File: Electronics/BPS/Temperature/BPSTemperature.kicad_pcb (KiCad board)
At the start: 2 copper layers, 75 x 65 mm, 59 parts, among them J1 Conn_02x10_Counter_Clockwise, J2 Logic Analyzer, J3 Conn_02x06_Counter_Clockwise, J4 Conn_02x06_Counter_Clockwise, SW1 SW_DIP_x06, U1 LTC2983

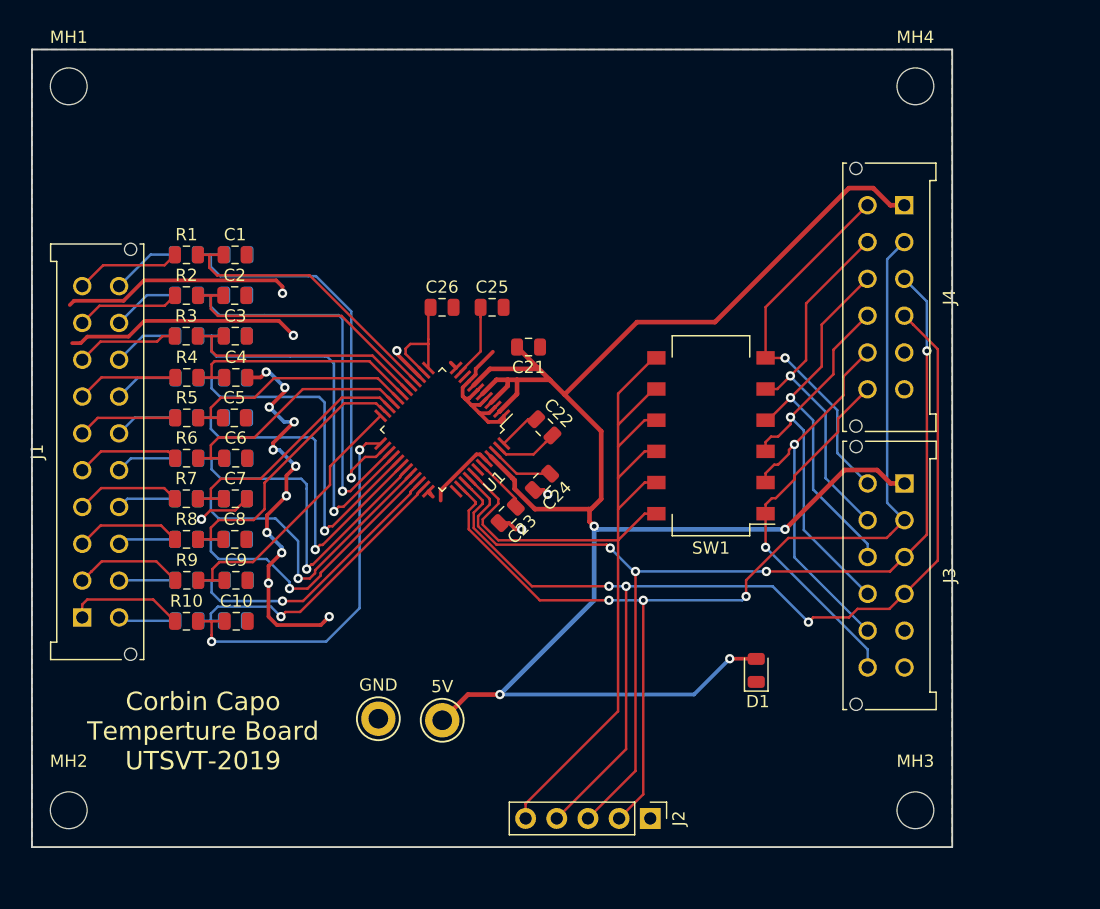
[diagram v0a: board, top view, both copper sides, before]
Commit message: Made edits to temperature board. Finalized boards.
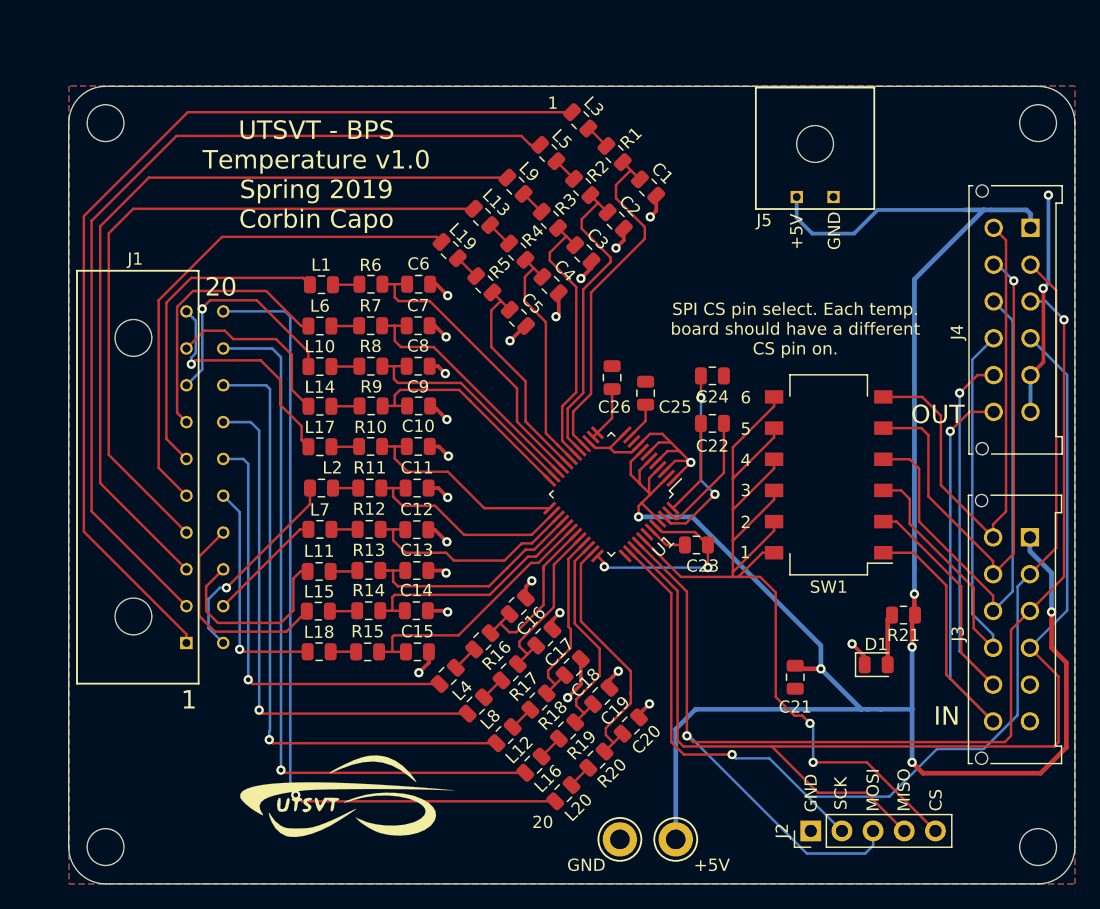
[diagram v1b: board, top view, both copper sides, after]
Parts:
- removed 5V: TestPoint, TestPoint:TestPoint_Keystone_5005-5009_Compact
- added +5V: TestPoint, TestPoint:TestPoint_Keystone_5005-5009_Compact, F.Cu at (102.5, 131.4)
- added G***: LOGO, UTSVT_Special:UTSVT_Logo_Symbol, F.Cu at (75.4, 128.0)
- added G***: LOGO, UTSVT_Special:Hallock_Image, B.Cu at (83.2, 100.8)
- added J5: Conn_01x02, UTSVT_Connectors:43650-0202_01x02_Microfit 3.0_horizontal, F.Cu at (109.0, 80.0)
- added L1: Ferrite_Bead, Inductor_SMD:L_0805_2012Metric, F.Cu at (73.6, 86.2)
- added L10: Ferrite_Bead, Inductor_SMD:L_0805_2012Metric, F.Cu at (73.5, 92.8)
- added L11: Ferrite_Bead, Inductor_SMD:L_0805_2012Metric, F.Cu at (73.4, 109.5)
- added L12: Ferrite_Bead, Inductor_SMD:L_0805_2012Metric, F.Cu at (88.5, 122.9)
- added L13: Ferrite_Bead, Inductor_SMD:L_0805_2012Metric, F.Cu at (86.7, 80.6)
- added L14: Ferrite_Bead, Inductor_SMD:L_0805_2012Metric, F.Cu at (73.5, 96.1)
- added L15: Ferrite_Bead, Inductor_SMD:L_0805_2012Metric, F.Cu at (73.3, 112.8)
- added L16: Ferrite_Bead, Inductor_SMD:L_0805_2012Metric, F.Cu at (90.9, 125.3)
- added L17: Ferrite_Bead, Inductor_SMD:L_0805_2012Metric, F.Cu at (73.5, 99.4)
- added L18: Ferrite_Bead, Inductor_SMD:L_0805_2012Metric, F.Cu at (73.4, 116.1)
- added L19: Ferrite_Bead, Inductor_SMD:L_0805_2012Metric, F.Cu at (84.0, 83.3)
- added L2: Ferrite_Bead, Inductor_SMD:L_0805_2012Metric, F.Cu at (73.6, 102.7)
- added L20: Ferrite_Bead, Inductor_SMD:L_0805_2012Metric, F.Cu at (93.3, 127.6)
- added L3: Ferrite_Bead, Inductor_SMD:L_0805_2012Metric, F.Cu at (94.7, 72.8)
- added L4: Ferrite_Bead, Inductor_SMD:L_0805_2012Metric, F.Cu at (83.9, 118.0)
- added L5: Ferrite_Bead, Inductor_SMD:L_0805_2012Metric, F.Cu at (92.1, 75.4)
- added L6: Ferrite_Bead, Inductor_SMD:L_0805_2012Metric, F.Cu at (73.5, 89.5)
- added L7: Ferrite_Bead, Inductor_SMD:L_0805_2012Metric, F.Cu at (73.5, 106.1)
- added L8: Ferrite_Bead, Inductor_SMD:L_0805_2012Metric, F.Cu at (86.2, 120.5)
- added L9: Ferrite_Bead, Inductor_SMD:L_0805_2012Metric, F.Cu at (89.4, 78.1)
- added R21: 1.55k, Resistor_SMD:R_0805_2012Metric, F.Cu at (121.0, 113.1)
- C11, C12, C13, C14, C15, C16, C17, C18, C19, C20, R11, R12, R13, R14, R15, R16, R17, R18, R19, R20: moved to F.Cu
- J1: footprint Connector_Molex:Molex_Micro-Fit_3.0_43045-2012_2x10_P3.00mm_Vertical -> UTSVT_Connectors:02x10_Microfit_3.0_horizontal
- moved R1 35.8 mm to (97.5, 75.5), turned to 315 degrees
- moved R20 35.2 mm to (96.0, 124.9), turned to 45 degrees
- moved C21 34.6 mm to (112.2, 118.2), turned to 90 degrees
- moved C1 34.1 mm to (100.2, 78.2), turned to 315 degrees
- moved R2 33.4 mm to (94.8, 78.2), turned to 315 degrees
- moved C20 33.3 mm to (98.8, 122.1), turned to 45 degrees
- moved R19 33.3 mm to (93.6, 122.5), turned to 45 degrees
- moved C2 31.6 mm to (97.6, 80.9), turned to 315 degrees
- moved R18 31.6 mm to (91.3, 120.1), turned to 45 degrees
- moved C19 31.2 mm to (96.4, 119.7), turned to 45 degrees
- moved R3 31.1 mm to (92.2, 80.9), turned to 315 degrees
- moved R17 29.9 mm to (88.9, 117.8), turned to 45 degrees
- moved C18 29.4 mm to (94.1, 117.3), turned to 45 degrees
- moved C3 29.2 mm to (94.9, 83.6), turned to 315 degrees
- moved R4 28.8 mm to (89.6, 83.5), turned to 315 degrees
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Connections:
- D1 pad 2: +5V -> Net-(D1-Pad2)
- J1 pad 1: /CH10_LPF -> /CH1_LPF
- J1 pad 10: /CH1_LPF -> /CH10_LPF
- J1 pad 11: /CH20_LPF -> /CH11_LPF
- J1 pad 12: /CH19_LPF -> /CH12_LPF
- J1 pad 13: /CH18_LPF -> /CH13_LPF
- J1 pad 14: /CH17_LPF -> /CH14_LPF
- J1 pad 15: /CH16_LPF -> /CH15_LPF
- J1 pad 16: /CH15_LPF -> /CH16_LPF
- J1 pad 17: /CH14_LPF -> /CH17_LPF
- J1 pad 18: /CH13_LPF -> /CH18_LPF
- J1 pad 19: /CH12_LPF -> /CH19_LPF
- J1 pad 2: /CH9_LPF -> /CH2_LPF
- J1 pad 20: /CH11_LPF -> /CH20_LPF
- J1 pad 3: /CH8_LPF -> /CH3_LPF
- J1 pad 4: /CH7_LPF -> /CH4_LPF
- J1 pad 5: /CH6_LPF -> /CH5_LPF
- J1 pad 6: /CH5_LPF -> /CH6_LPF
- J1 pad 7: /CH4_LPF -> /CH7_LPF
- J1 pad 8: /CH3_LPF -> /CH8_LPF
- J1 pad 9: /CH2_LPF -> /CH9_LPF
- R1 pad 1: /CH1_LPF -> Net-(L3-Pad1)
- R10 pad 1: /CH10_LPF -> Net-(L17-Pad1)
- R11 pad 1: /CH11_LPF -> Net-(L2-Pad2)
- R12 pad 1: /CH12_LPF -> Net-(L7-Pad2)
- R13 pad 1: /CH13_LPF -> Net-(L11-Pad2)
- R14 pad 1: /CH14_LPF -> Net-(L15-Pad2)
- R15 pad 1: /CH15_LPF -> Net-(L18-Pad2)
- R16 pad 1: /CH16_LPF -> Net-(L4-Pad2)
- R17 pad 1: /CH17_LPF -> Net-(L8-Pad2)
- R18 pad 1: /CH18_LPF -> Net-(L12-Pad2)
- R19 pad 1: /CH19_LPF -> Net-(L16-Pad2)
- R2 pad 1: /CH2_LPF -> Net-(L5-Pad1)
- R20 pad 1: /CH20_LPF -> Net-(L20-Pad2)
- R3 pad 1: /CH3_LPF -> Net-(L9-Pad1)
- R4 pad 1: /CH4_LPF -> Net-(L13-Pad1)
- R5 pad 1: /CH5_LPF -> Net-(L19-Pad1)
- R6 pad 1: /CH6_LPF -> Net-(L1-Pad2)
- R7 pad 1: /CH7_LPF -> Net-(L6-Pad2)
- R8 pad 1: /CH8_LPF -> Net-(L10-Pad2)
- R9 pad 1: /CH9_LPF -> Net-(L14-Pad2)
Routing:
- net /CH1_LPF: track 8.61 -> 81.5 mm
- net /CH2_LPF: track 8.48 -> 74.3 mm
- net /CH20_LPF: track 4.71 -> 66.2 mm, vias 0 -> 1
- net /CH3_LPF: track 8.33 -> 65.7 mm
- net /CH19_LPF: track 4.57 -> 58.7 mm, vias 0 -> 1
- net /CH4_LPF: track 8.23 -> 57.6 mm
- net /CH18_LPF: track 4.71 -> 51.2 mm, vias 0 -> 1
- net /CH17_LPF: track 4.82 -> 43.1 mm, vias 0 -> 1
- net /CH5_LPF: track 8.10 -> 42.2 mm
- net /CH16_LPF: track 4.99 -> 35.5 mm, vias 0 -> 1
- net +5V: track 153.5 -> 176.2 mm, vias 4 -> 6
- net /CS1: track 29.7 -> 48.2 mm
- net /CH6_LPF: track 8.43 -> 26.2 mm
- net /MOSI: track 87.7 -> 103.9 mm, vias 4 -> 2
- net Net-(C11-Pad1): track 33.8 -> 17.8 mm, vias 1 -> 0
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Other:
- board size 75 x 65 mm -> 82 x 65 mm
- rule pad_to_mask_clearance: 0.2 -> 0
- rule via_min_drill: 0.254 -> 0.3
- rule via_min_size: 0.381 -> 0.508
- board text added: "+5V"
- board text added: "1"
- board text added: "2"
- board text added: "20"
- board text added: "3"
- board text added: "4"
- board text added: "5"
- board text added: "6"
- board text added: "CS"
- board text added: "GND"
- board text added: "IN"
- board text added: "MISO"
- board text added: "MOSI"
- board text added: "OUT"
- board text added: "SCK"
- board text added: "SPI CS pin select. Each temp. board should have a different CS pin on."
- board text added: "Spring 2019: Monolo Alvarez Chase Block Corbin Capo Richard Li Austin Tsao Garrett Wong Sihyung Woo Sijin Woo"
- board text added: "UTSVT - BPS Temperature v1.0 Spring 2019 Corbin Capo"
- board text removed: "Corbin Capo Temperture Board UTSVT-2019"
